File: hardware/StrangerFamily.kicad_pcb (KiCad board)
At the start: 2 copper layers, 85 x 47 mm, 23 parts, among them J1 LCD_Conn, J2 Power_LEDs, J3 Output_LED, J5 Raspberry_Pi_zero, Q1 BSS138, Q2 BSS138, Q3 BSS138, Q4 BSS138

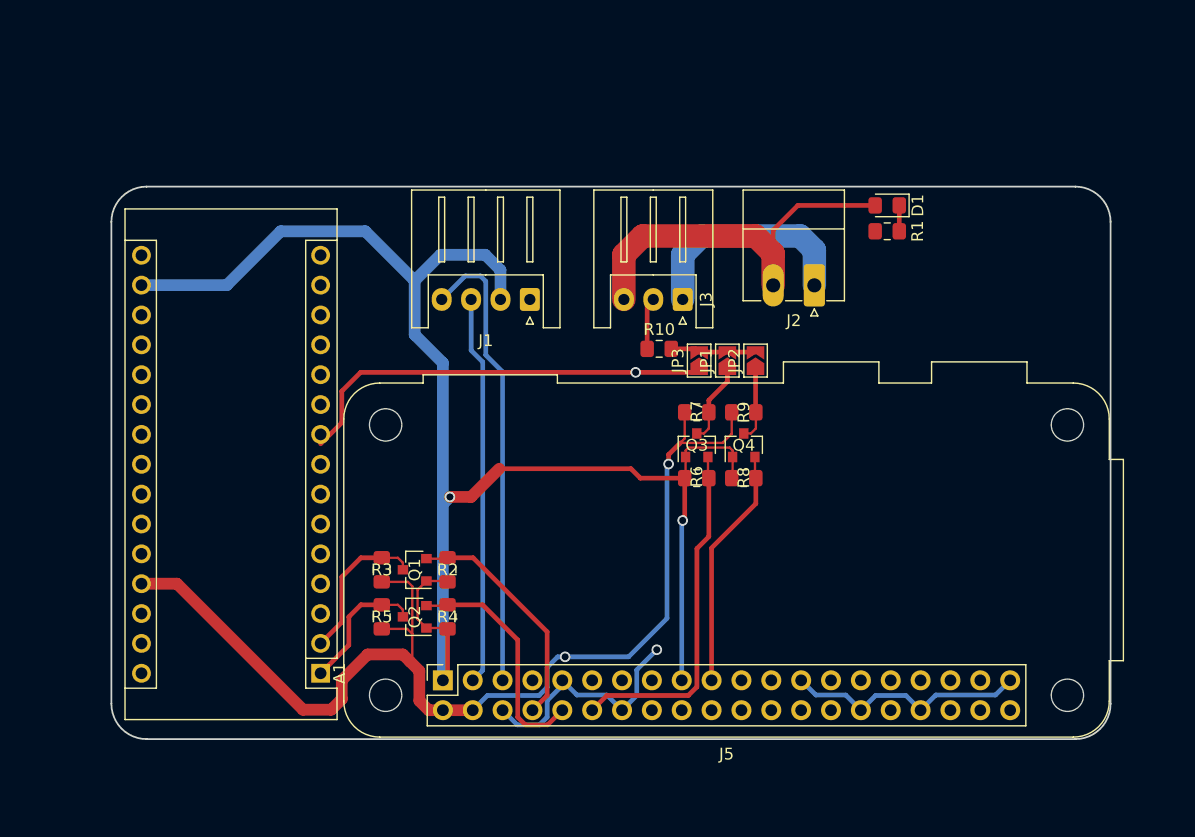
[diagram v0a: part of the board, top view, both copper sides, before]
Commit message: Update hardware designs. This is v2 sent to prod in august 2020.
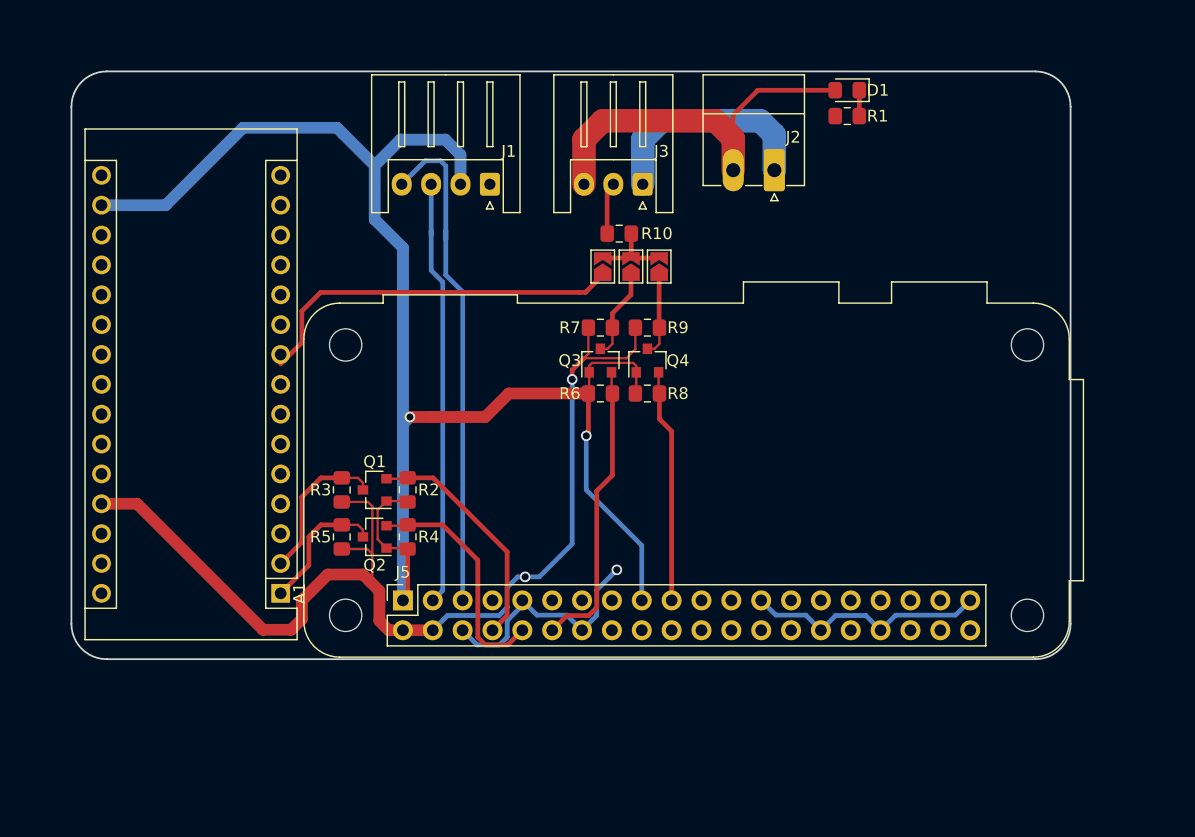
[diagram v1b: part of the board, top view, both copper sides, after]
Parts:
- moved JP1 11.5 mm to (217.6, 86.6)
- moved JP3 11.5 mm to (215.2, 86.6)
- moved JP2 11.5 mm to (220.0, 86.6)
- moved Q3 10.9 mm to (215.0, 94.6)
- moved Q4 10.9 mm to (219.0, 94.6)
- moved R7 10.9 mm to (215.0, 91.8)
- moved R9 10.9 mm to (219.0, 91.8)
- moved R6 10.9 mm to (215.0, 97.4)
- moved R8 10.9 mm to (219.0, 97.4)
- moved D1 10.4 mm to (236.0, 71.6)
- moved J1 10.4 mm to (205.6, 79.6)
- moved J3 10.4 mm to (218.6, 79.6)
- moved R1 10.4 mm to (236.0, 73.8)
- moved R10 10.4 mm to (216.6, 83.8)
- moved J2 10.4 mm to (229.8, 78.4)
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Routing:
- net /PWM0: track 29.7 -> 25.2 mm
- net /Arduino_out: track 36.4 -> 32.1 mm, vias 1 -> 0
- net +5V: track 96.4 -> 92.5 mm
- net /LCD_SLC: track 39.3 -> 43.1 mm
- net /LCD_SDA: track 33.2 -> 36.5 mm
- net /MOSI_5V: track 6.26 -> 7.06 mm
- net /PWM0_5V: track 6.90 -> 7.70 mm
- net /MOSI: track 20.6 -> 19.9 mm
- net +3V3: track 134.4 -> 134.9 mm
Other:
- board size 85 x 47 mm -> 85 x 50 mm
